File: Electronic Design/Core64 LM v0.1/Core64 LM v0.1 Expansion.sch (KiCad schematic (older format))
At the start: 7 parts

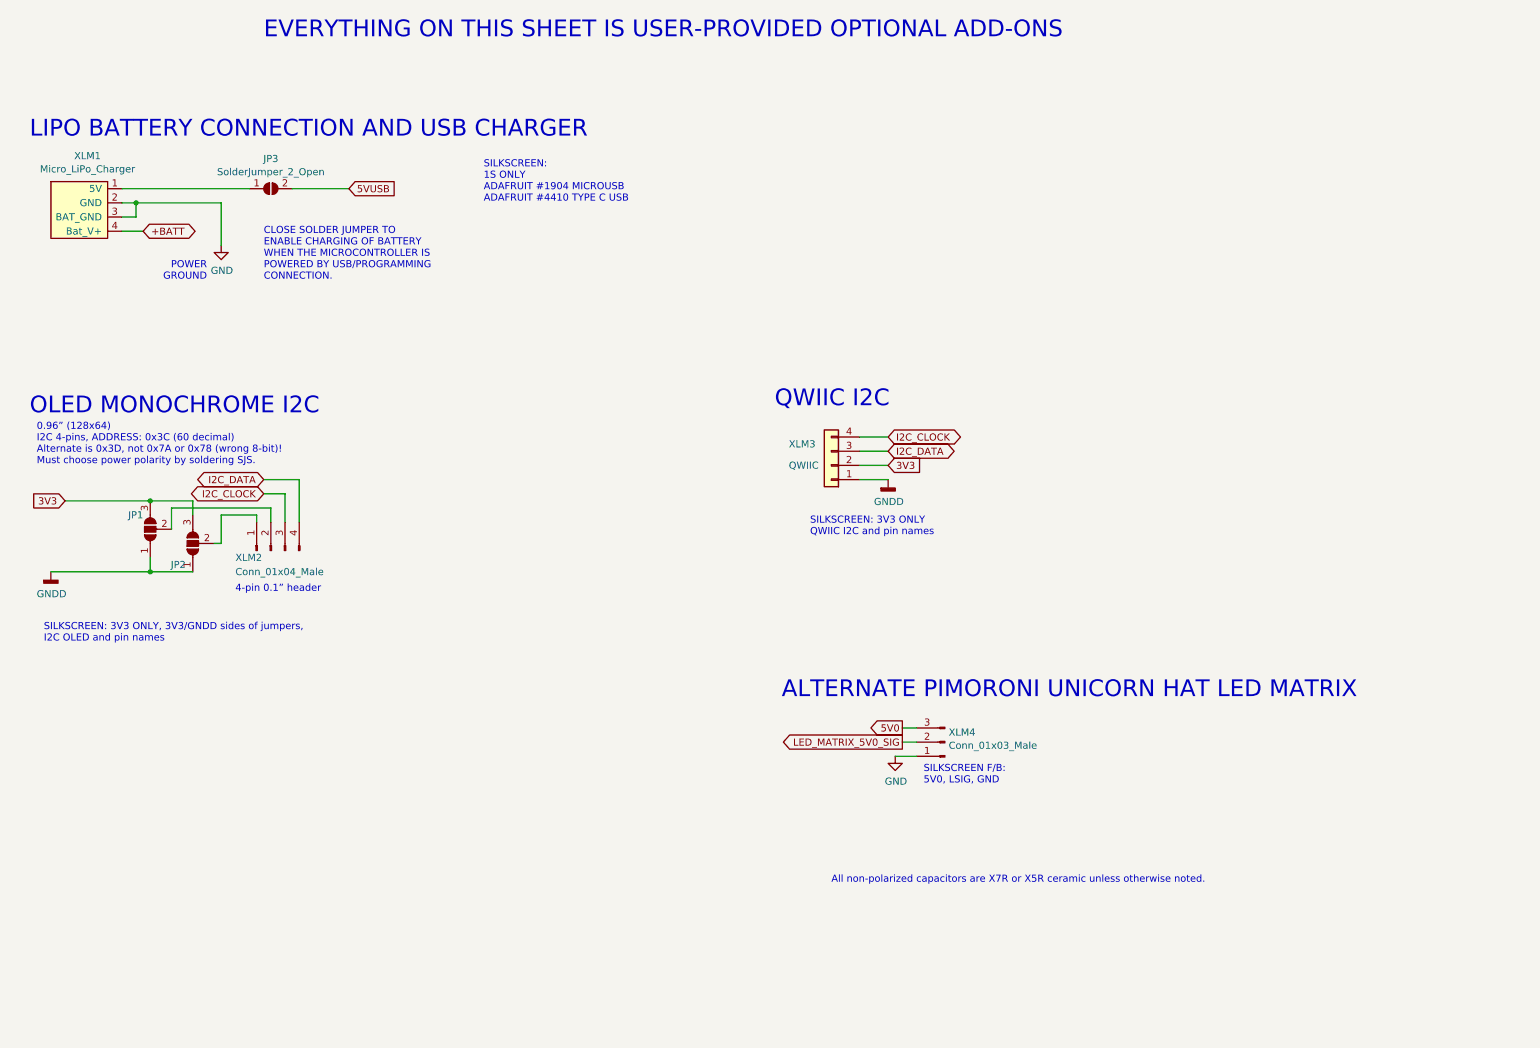
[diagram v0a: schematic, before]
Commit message: Finish layout, revise notes
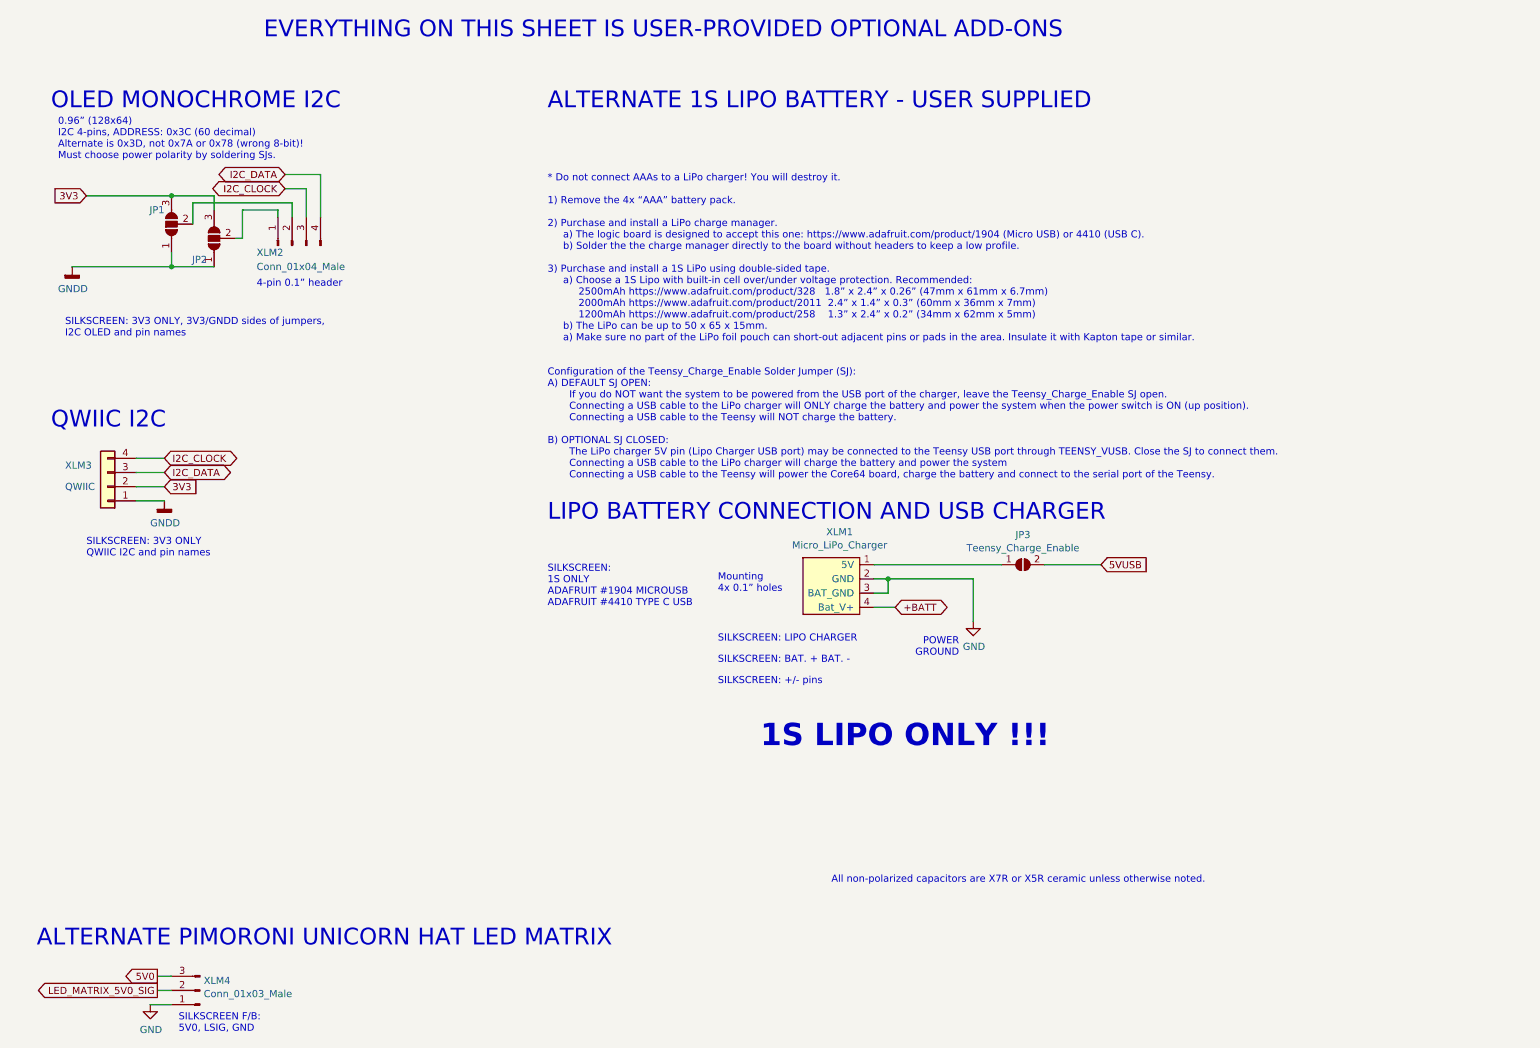
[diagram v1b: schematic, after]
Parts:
- JP3: value SolderJumper_2_Open -> Teensy_Charge_Enable
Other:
- note added: "* Do not connect AAAs to a LiPo charger! You will destroy it.\n\n1) Remove the 4x “AAA” battery pack.\n\n2) Purchase and install a LiPo charge manager.\n a) The logic board is designed to accept this one: https://www.adafruit.com/product/1904 (Micro USB) or 4410 (USB C).\n b) Solder the the charge manager directly to the board without headers to keep a low profile.\n\n3) Purchase and install a 1S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"
- note added: "0.96” (128x64)\nI2C 4-pins, ADDRESS: 0x3C (60 decimal)\nAlternate is 0x3D, not 0x7A or 0x78 (wrong 8-bit)!\nMust choose power polarity by soldering SJs."
- note added: "1S LIPO ONLY !!!"
- note added: "ALTERNATE 1S LIPO BATTERY - USER SUPPLIED"
- note added: "Mounting\n4x 0.1” holes"
- note added: "SILKSCREEN: +/- pins"
- note added: "SILKSCREEN: BAT. + BAT. -"
- note added: "SILKSCREEN: LIPO CHARGER"
- note removed: "0.96” (128x64)\nI2C 4-pins, ADDRESS: 0x3C (60 decimal)\nAlternate is 0x3D, not 0x7A or 0x78 (wrong 8-bit)!\nMust choose power polarity by soldering SJS."
- note removed: "CLOSE SOLDER JUMPER TO\nENABLE CHARGING OF BATTERY\nWHEN THE MICROCONTROLLER IS\nPOWERED BY USB/PROGRAMMING\nCONNECTION."
- moved on the sheet: JP1, JP2, JP3, XLM1, XLM2, XLM3, XLM4
